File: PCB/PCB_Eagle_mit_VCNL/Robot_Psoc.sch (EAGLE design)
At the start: 178 parts, among them IC1 LD117AS33TR, U1 CY8C4247AZI-M485, U2 VCNL4010-GS08, U3 VCNL4010-GS08, U4 VCNL4010-GS08, U5 VCNL4010-GS08, X1 FH12-10S-0.5SH, X2 FH12-10S-0.5SH

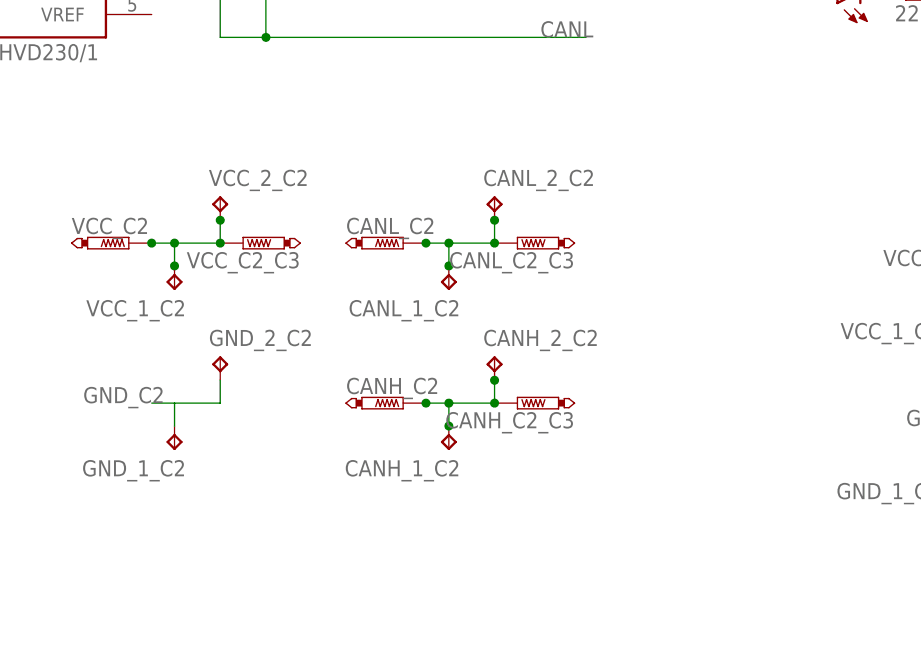
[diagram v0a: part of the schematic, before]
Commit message: 15/11/2016
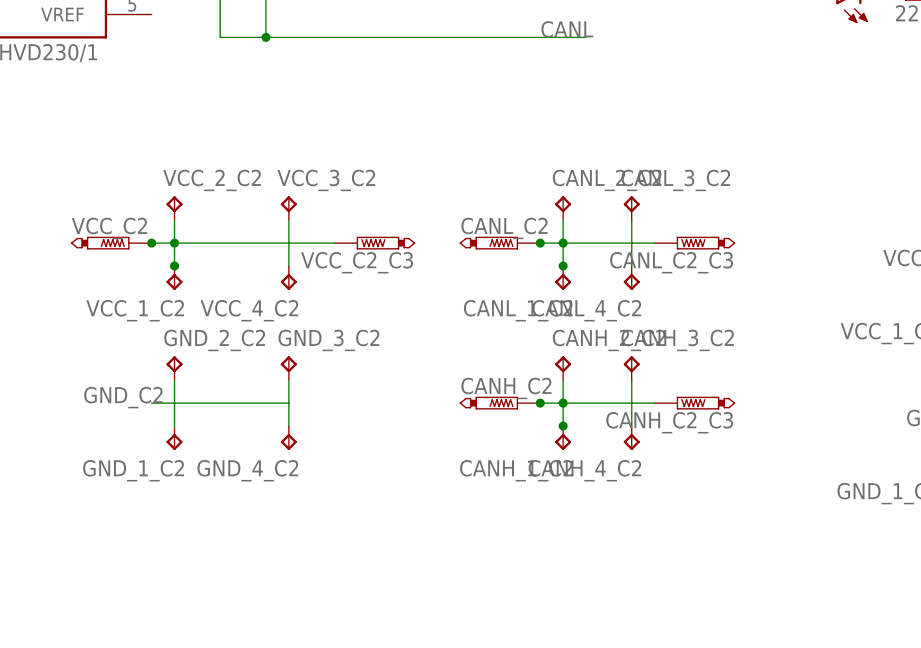
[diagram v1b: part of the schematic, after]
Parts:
- added CANH_3_C2, CANH_4_C2, CANL_3_C2, CANL_4_C2, GND_3_C2, GND_4_C2, VCC_3_C2, VCC_4_C2: TPB2,54, testpad:TPB2,54
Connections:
- net GND_C2: now also GND_3_C2.TP, GND_4_C2.TP
- net N$32: now also CANL_3_C2.TP, CANL_4_C2.TP
- net N$7: now also CANH_3_C2.TP, CANH_4_C2.TP
- net VCC_C2: now also VCC_3_C2.TP, VCC_4_C2.TP
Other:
- moved on the sheet: CANH_1_C2, CANH_2_C2, CANH_C2, CANH_C2_C3, CANL_1_C2, CANL_2_C2, CANL_C2, CANL_C2_C3, GND_2_C2, VCC_2_C2, VCC_C2_C3
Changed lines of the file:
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@@
 <part name="R26" library="rcl" deviceset="R-EU_" device="R0805" value="4.7k"/>
 <part name="R27" library="rcl" deviceset="R-EU_" device="R0805" value="4.7k"/>
+<part name="GND_4_C2" library="testpad" deviceset="TP" device="B2,54"/>
+<part name="GND_3_C2" library="testpad" deviceset="TP" device="B2,54"/>
+<part name="VCC_3_C2" library="testpad" deviceset="TP" device="B2,54"/>
+<part name="VCC_4_C2" library="testpad" deviceset="TP" device="B2,54"/>
+<part name="CANL_4_C2" library="testpad" deviceset="TP" device="B2,54"/>
+<part name="CANL_3_C2" library="testpad" deviceset="TP" device="B2,54"/>
+<part name="CANH_4_C2" library="testpad" deviceset="TP" device="B2,54"/>
+<part name="CANH_3_C2" library="testpad" deviceset="TP" device="B2,54"/>
 </parts>
 <sheets>
@@
 <instance part="CANH_4_C1" gate="G$1" x="96.52" y="-66.04"/>
 <instance part="CANH_C1" gate="G$1" x="73.66" y="-71.12" rot="R270"/>
-<instance part="VCC_2_C2" gate="G$1" x="142.24" y="-48.26"/>
+<instance part="VCC_2_C2" gate="G$1" x="137.16" y="-48.26"/>
 <instance part="VCC_1_C2" gate="G$1" x="137.16" y="-58.42" rot="R180"/>
 <instance part="VCC_C2" gate="G$1" x="132.08" y="-53.34" rot="R270"/>
-<instance part="GND_2_C2" gate="G$1" x="142.24" y="-66.04"/>
+<instance part="GND_2_C2" gate="G$1" x="137.16" y="-66.04"/>
 <instance part="GND_1_C2" gate="G$1" x="137.16" y="-76.2" rot="R180"/>
-<instance part="CANL_2_C2" gate="G$1" x="172.72" y="-48.26"/>
-<instance part="CANL_1_C2" gate="G$1" x="167.64" y="-58.42" rot="R180"/>
-<instance part="CANL_C2" gate="G$1" x="162.56" y="-53.34" rot="R270"/>
-<instance part="CANH_2_C2" gate="G$1" x="172.72" y="-66.04"/>
-<instance part="CANH_1_C2" gate="G$1" x="167.64" y="-76.2" rot="R180"/>
-<instance part="CANH_C2" gate="G$1" x="162.56" y="-71.12" rot="R270"/>
+<instance part="CANL_2_C2" gate="G$1" x="180.34" y="-48.26"/>
+<instance part="CANL_1_C2" gate="G$1" x="180.34" y="-58.42" rot="R180"/>
+<instance part="CANL_C2" gate="G$1" x="175.26" y="-53.34" rot="R270"/>
+<instance part="CANH_2_C2" gate="G$1" x="180.34" y="-66.04"/>
+<instance part="CANH_1_C2" gate="G$1" x="180.34" y="-76.2" rot="R180"/>
+<instance part="CANH_C2" gate="G$1" x="175.26" y="-71.12" rot="R270"/>
 <instance part="VCC_2_C3" gate="G$1" x="226.06" y="-50.8"/>
 <instance part="VCC_1_C3" gate="G$1" x="220.98" y="-60.96" rot="R180"/>
@@
 <instance part="CANH_3_C4" gate="G$1" x="373.38" y="-78.74" rot="R180"/>
 <instance part="CANH_4_C4" gate="G$1" x="378.46" y="-68.58"/>
-<instance part="VCC_C2_C3" gate="G$1" x="144.78" y="-53.34" rot="R90"/>
-<instance part="CANL_C2_C3" gate="G$1" x="175.26" y="-53.34" rot="R90"/>
-<instance part="CANH_C2_C3" gate="G$1" x="175.26" y="-71.12" rot="R90"/>
+<instance part="VCC_C2_C3" gate="G$1" x="157.48" y="-53.34" rot="R90"/>
+<instance part="CANL_C2_C3" gate="G$1" x="193.04" y="-53.34" rot="R90"/>
+<instance part="CANH_C2_C3" gate="G$1" x="193.04" y="-71.12" rot="R90"/>
 <instance part="MECH_LINK_1" gate="G$1" x="363.22" y="-20.32" rot="R270"/>
 <instance part="MECH_LINK_2" gate="G$1" x="363.22" y="-25.4" rot="R270"/>
@@
 <instance part="R26" gate="G$1" x="210.82" y="-10.16" rot="R270"/>
 <instance part="R27" gate="G$1" x="218.44" y="-10.16" rot="R270"/>
+<instance part="GND_4_C2" gate="G$1" x="149.86" y="-76.2" rot="R180"/>
+<instance part="GND_3_C2" gate="G$1" x="149.86" y="-66.04"/>
+<instance part="VCC_3_C2" gate="G$1" x="149.86" y="-48.26"/>
+<instance part="VCC_4_C2" gate="G$1" x="149.86" y="-58.42" rot="R180"/>
+<instance part="CANL_4_C2" gate="G$1" x="187.96" y="-58.42" rot="R180"/>
+<instance part="CANL_3_C2" gate="G$1" x="187.96" y="-48.26"/>
+<instance part="CANH_4_C2" gate="G$1" x="187.96" y="-76.2" rot="R180"/>
+<instance part="CANH_3_C2" gate="G$1" x="187.96" y="-66.04"/>
 </instances>
 <busses>
@@
 <wire x1="137.16" y1="-73.66" x2="137.16" y2="-71.12" width="0.1524" layer="91"/>
 <pinref part="GND_2_C2" gate="G$1" pin="TP"/>
-<wire x1="137.16" y1="-71.12" x2="142.24" y2="-71.12" width="0.1524" layer="91"/>
-<wire x1="142.24" y1="-68.58" x2="142.24" y2="-71.12" width="0.1524" layer="91"/>
+<wire x1="137.16" y1="-68.58" x2="137.16" y2="-71.12" width="0.1524" layer="91"/>
 <label x="127" y="-71.12" size="1.778" layer="95"/>
+<pinref part="GND_4_C2" gate="G$1" pin="TP"/>
+<wire x1="149.86" y1="-73.66" x2="149.86" y2="-71.12" width="0.1524" layer="91"/>
+<wire x1="149.86" y1="-71.12" x2="137.16" y2="-71.12" width="0.1524" layer="91"/>
+<pinref part="GND_3_C2" gate="G$1" pin="TP"/>
+<wire x1="149.86" y1="-68.58" x2="149.86" y2="-71.12" width="0.1524" layer="91"/>
 </segment>
 <segment>
@@
 <wire x1="134.62" y1="-53.34" x2="137.16" y2="-53.34" width="0.1524" layer="91"/>
 <wire x1="137.16" y1="-53.34" x2="137.16" y2="-55.88" width="0.1524" layer="91"/>
-<pinref part="VCC_2_C2" gate="G$1" pin="TP"/>
-<wire x1="142.24" y1="-50.8" x2="142.24" y2="-53.34" width="0.1524" layer="91"/>
-<wire x1="142.24" y1="-53.34" x2="137.16" y2="-53.34" width="0.1524" layer="91"/>
+<wire x1="154.94" y1="-53.34" x2="149.86" y2="-53.34" width="0.1524" layer="91"/>
 <junction x="134.62" y="-53.34"/>
 <junction x="137.16" y="-55.88"/>
-<junction x="142.24" y="-50.8"/>
 <junction x="137.16" y="-53.34"/>
 <pinref part="VCC_C2_C3" gate="G$1" pin="TP"/>
-<junction x="142.24" y="-53.34"/>
+<pinref part="VCC_2_C2" gate="G$1" pin="TP"/>
+<wire x1="149.86" y1="-53.34" x2="137.16" y2="-53.34" width="0.1524" layer="91"/>
+<wire x1="137.16" y1="-50.8" x2="137.16" y2="-53.34" width="0.1524" layer="91"/>
+<pinref part="VCC_4_C2" gate="G$1" pin="TP"/>
+<wire x1="149.86" y1="-55.88" x2="149.86" y2="-53.34" width="0.1524" layer="91"/>
+<pinref part="VCC_3_C2" gate="G$1" pin="TP"/>
+<wire x1="149.86" y1="-50.8" x2="149.86" y2="-53.34" width="0.1524" layer="91"/>
 </segment>
 <segment>
@@
 <pinref part="CANL_C2" gate="G$1" pin="TP"/>
 <pinref part="CANL_1_C2" gate="G$1" pin="TP"/>
-<wire x1="165.1" y1="-53.34" x2="167.64" y2="-53.34" width="0.1524" layer="91"/>
-<wire x1="167.64" y1="-53.34" x2="167.64" y2="-55.88" width="0.1524" layer="91"/>
+<wire x1="177.8" y1="-53.34" x2="180.34" y2="-53.34" width="0.1524" layer="91"/>
+<wire x1="180.34" y1="-53.34" x2="180.34" y2="-55.88" width="0.1524" layer="91"/>
+<wire x1="190.5" y1="-53.34" x2="187.96" y2="-53.34" width="0.1524" layer="91"/>
+<junction x="177.8" y="-53.34"/>
+<junction x="180.34" y="-55.88"/>
+<junction x="180.34" y="-53.34"/>
+<pinref part="CANL_C2_C3" gate="G$1" pin="TP"/>
 <pinref part="CANL_2_C2" gate="G$1" pin="TP"/>
-<wire x1="172.72" y1="-50.8" x2="172.72" y2="-53.34" width="0.1524" layer="91"/>
-<wire x1="172.72" y1="-53.34" x2="167.64" y2="-53.34" width="0.1524" layer="91"/>
-<junction x="165.1" y="-53.34"/>
-<junction x="167.64" y="-55.88"/>
-<junction x="172.72" y="-50.8"/>
-<junction x="167.64" y="-53.34"/>
-<pinref part="CANL_C2_C3" gate="G$1" pin="TP"/>
-<junction x="172.72" y="-53.34"/>
+<wire x1="187.96" y1="-53.34" x2="180.34" y2="-53.34" width="0.1524" layer="91"/>
+<wire x1="180.34" y1="-50.8" x2="180.34" y2="-53.34" width="0.1524" layer="91"/>
+<pinref part="CANL_3_C2" gate="G$1" pin="TP"/>
+<wire x1="187.96" y1="-50.8" x2="187.96" y2="-53.34" width="0.1524" layer="91"/>
+<pinref part="CANL_4_C2" gate="G$1" pin="TP"/>
+<wire x1="187.96" y1="-55.88" x2="187.96" y2="-53.34" width="0.1524" layer="91"/>
 </segment>
 </net>
@@
 <pinref part="CANH_C2" gate="G$1" pin="TP"/>
 <pinref part="CANH_1_C2" gate="G$1" pin="TP"/>
-<wire x1="165.1" y1="-71.12" x2="167.64" y2="-71.12" width="0.1524" layer="91"/>
-<wire x1="167.64" y1="-73.66" x2="167.64" y2="-71.12" width="0.1524" layer="91"/>
-<wire x1="167.64" y1="-71.12" x2="172.72" y2="-71.12" width="0.1524" layer="91"/>
+<wire x1="177.8" y1="-71.12" x2="180.34" y2="-71.12" width="0.1524" layer="91"/>
+<wire x1="180.34" y1="-73.66" x2="180.34" y2="-71.12" width="0.1524" layer="91"/>
+<wire x1="180.34" y1="-71.12" x2="187.96" y2="-71.12" width="0.1524" layer="91"/>
+<junction x="177.8" y="-71.12"/>
+<junction x="180.34" y="-73.66"/>
+<junction x="180.34" y="-71.12"/>
+<pinref part="CANH_C2_C3" gate="G$1" pin="TP"/>
 <pinref part="CANH_2_C2" gate="G$1" pin="TP"/>
-<wire x1="172.72" y1="-68.58" x2="172.72" y2="-71.12" width="0.1524" layer="91"/>
-<junction x="165.1" y="-71.12"/>
-<junction x="167.64" y="-73.66"/>
-<junction x="167.64" y="-71.12"/>
-<junction x="172.72" y="-68.58"/>
-<pinref part="CANH_C2_C3" gate="G$1" pin="TP"/>
-<junction x="172.72" y="-71.12"/>
-</segment>
-</net>
+<wire x1="187.96" y1="-71.12" x2="190.5" y2="-71.12" width="0.1524" layer="91"/>
+<wire x1="180.34" y1="-68.58" x2="180.34" y2="-71.12" width="0.1524" layer="91"/>
+<pinref part="CANH_3_C2" gate="G$1" pin="TP"/>
+<wire x1="187.96" y1="-68.58" x2="187.96" y2="-71.12" width="0.1524" layer="91"/>
+<pinref part="CANH_4_C2" gate="G$1" pin="TP"/>
+<wire x1="187.96" y1="-73.66" x2="187.96" y2="-71.12" width="0.1524" layer="91"/>
+</segment>
+</net>
